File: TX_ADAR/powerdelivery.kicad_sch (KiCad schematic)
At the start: 10 parts, among them U1 LT1761-1.8, U3 LT1761-2.5

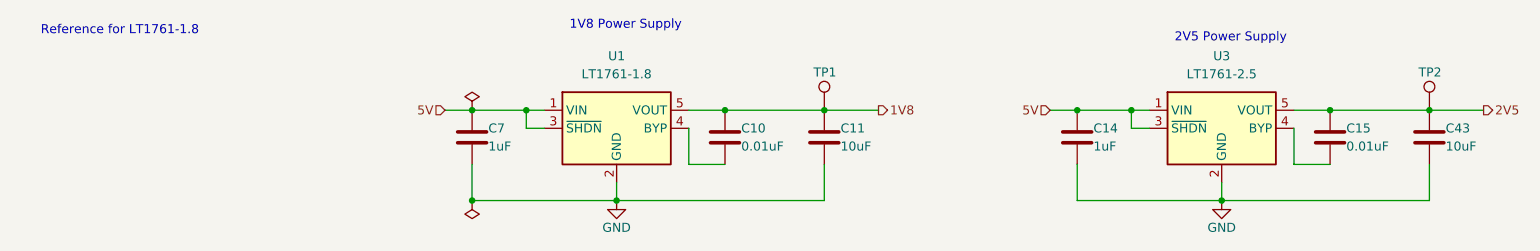
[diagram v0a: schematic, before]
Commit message: Fixing problems pointed out
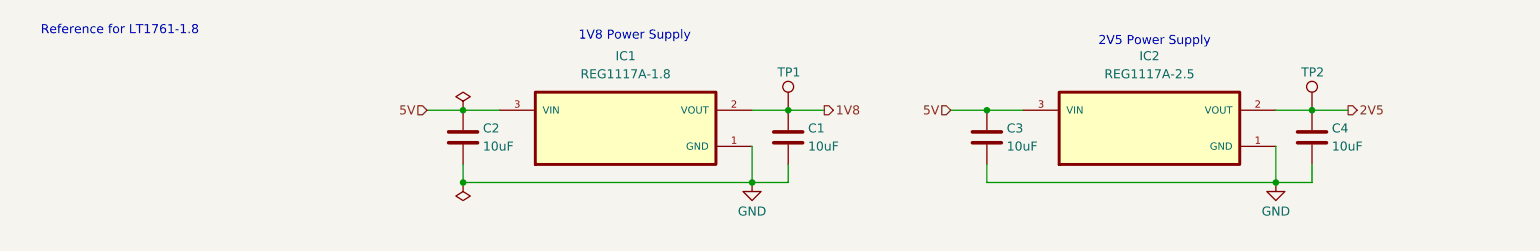
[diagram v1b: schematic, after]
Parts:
- removed C10, C15: 0.01uF, symbol Device:C
- removed C11, C43: 10uF, symbol Device:C
- removed C14, C7: 1uF, symbol Device:C
- removed U1: LT1761-1.8, Package_TO_SOT_SMD:TSOT-23-5, symbol Regulator_Linear:LT1761-1.8
- removed U3: LT1761-2.5, Package_TO_SOT_SMD:TSOT-23-5, symbol Regulator_Linear:LT1761-2.5
- added C1, C2, C3, C4: 10uF, Package_SO:SOIC-8_3.9x4.9mm_P1.27mm, symbol Device:C
- added IC1: REG1117A-1.8, Package_DFN_QFN:DFN-6-1EP_3x3mm_P0.95mm_EP1.7x2.6mm, symbol REG1117A-1.8:REG1117A-1.8
- added IC2: REG1117A-2.5, Package_DFN_QFN:DFN-6-1EP_3x3mm_P0.95mm_EP1.7x2.6mm, symbol REG1117A-2.5:REG1117A-2.5
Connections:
- net 1V8: now also C1.1, IC1.2 (VOUT)
- net 2V5: now also C4.1, IC2.2 (VOUT)
- net 5V: now also C2.1, C3.1, IC1.3 (VIN), IC2.3 (VIN)
- net GND: now also C1.2, C2.2, C3.2, C4.2, IC1.1 (GND), IC2.1 (GND)
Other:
- moved on the sheet: TP1, TP2
